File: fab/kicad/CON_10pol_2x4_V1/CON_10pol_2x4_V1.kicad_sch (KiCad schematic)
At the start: 7 parts, among them J1 Box_02x05_P2.54_Vertical, J2 Conn_01x04, J3 Conn_01x04

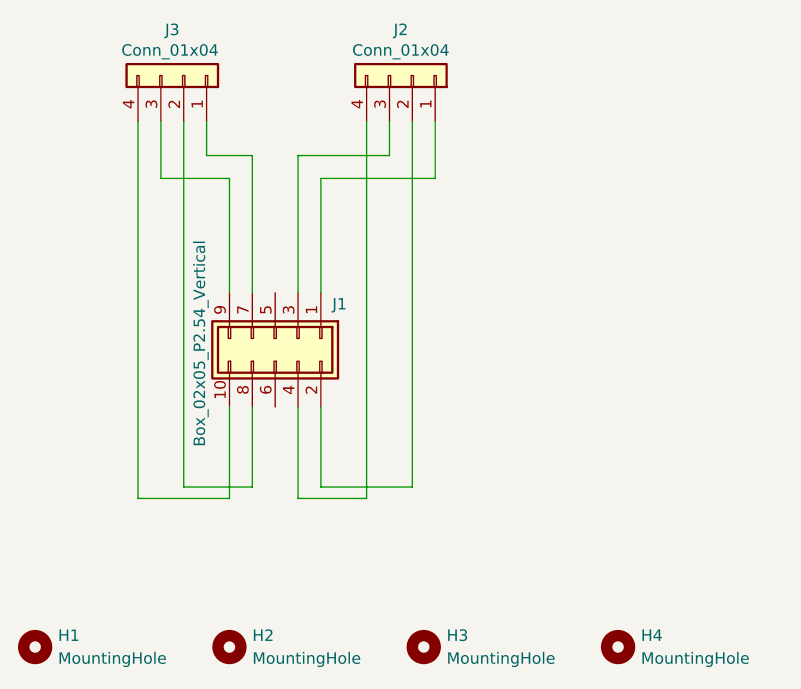
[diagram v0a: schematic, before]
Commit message: Update kicad-Files
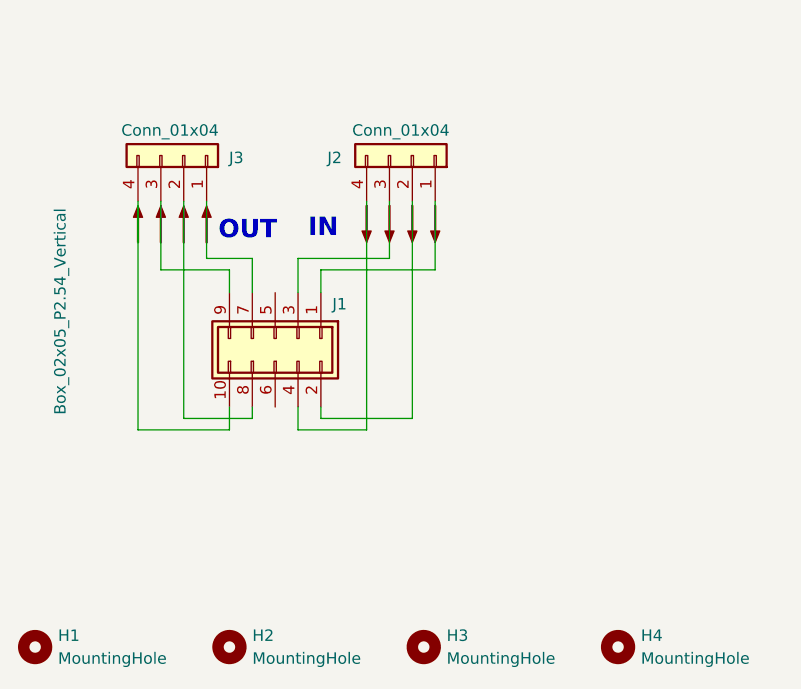
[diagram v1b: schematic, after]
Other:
- note added: "IN"
- note added: "OUT"
- moved on the sheet: J2, J3
